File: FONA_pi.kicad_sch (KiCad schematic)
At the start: 31 parts, among them J1 Conn_01x20_Socket, J10 Conn_01x04_Pin, J11 Conn_01x20_Socket, J12 Conn_01x20_Socket, J13 Conn_01x06_Socket, J14 Conn_01x06_Socket, J15 Conn_01x06_Socket, J16 Conn_01x06_Socket, J17 Conn_01x06_Socket, J18 Conn_01x04, J2 Conn_02x20_Odd_Even, J3 Conn_01x20_Socket, J4 Conn_01x20_Socket, J5 Conn_01x18, J6 Conn_01x18_Socket, J7 Conn_01x20_Socket, J8 Conn_01x18, J9 Conn_01x04_Pin

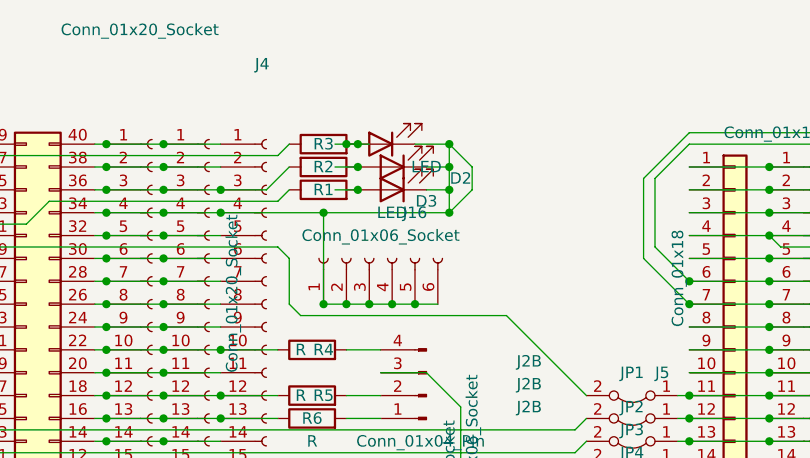
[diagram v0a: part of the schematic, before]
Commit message: Placed footprints again.
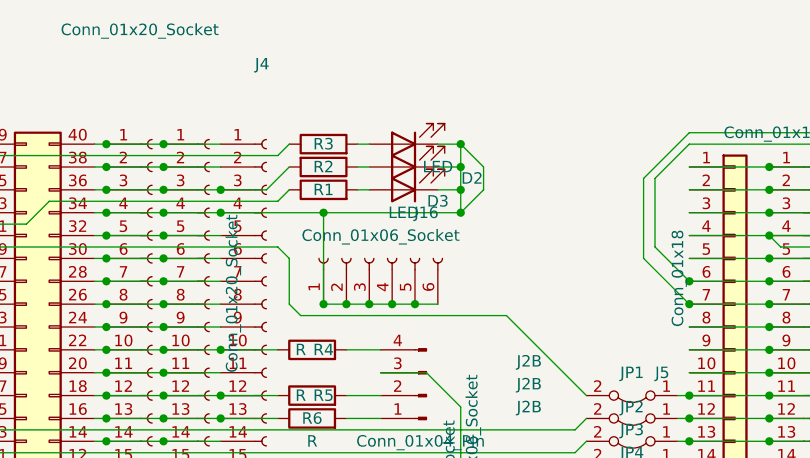
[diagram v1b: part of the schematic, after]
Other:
- moved on the sheet: D2, D3
